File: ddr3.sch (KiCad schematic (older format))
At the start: 17 parts

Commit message: add ddr3
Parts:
- added C? (x7): 0.22u, symbol C
- added C?: 22u, symbol C
- added C? (x4): 2.2p, symbol C
- added R?: 240, symbol R
- added R?: 470, symbol R
- added TP? (x2): A0, symbol TESTPOINT
- added TP? (x2): DQ0, symbol TESTPOINT
- added TP? (x2): CK, symbol TESTPOINT
- added TP? (x2): ~CK, symbol TESTPOINT
- added TP? (x4): GND, symbol TESTPOINT
- added U?: MT41K256M16-107, symbol DDR3-96FBGA
- R?: value Rs -> 10k; symbol Rs -> R
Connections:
- net labels added: DRAM_A0, DRAM_A1, DRAM_A10, DRAM_A11, DRAM_A12, DRAM_A13, DRAM_A14, DRAM_A2, DRAM_A3, DRAM_A4, DRAM_A5, DRAM_A6, DRAM_A7, DRAM_A8, DRAM_A9, DRAM_A[14:0],DRAM_BA[2:0],DRAM_CONTROL, DRAM_BA0, DRAM_BA1, DRAM_BA2, DRAM_CK, DRAM_CKE, DRAM_DATA[15:0],DRAM_DQ,DRAM_DM, DRAM_DQ0, DRAM_DQ1, DRAM_DQ10, DRAM_DQ11, DRAM_DQ12, DRAM_DQ13, DRAM_DQ14, DRAM_DQ15, DRAM_DQ2, DRAM_DQ3, DRAM_DQ4, DRAM_DQ5, DRAM_DQ6, DRAM_DQ7, DRAM_DQ8, DRAM_DQ9, DRAM_LDM, DRAM_LDQS, DRAM_ODT, DRAM_UDM, DRAM_UDQS, ~DRAM_CAS, ~DRAM_CK, ~DRAM_CS, ~DRAM_LDQS, ~DRAM_RAS, ~DRAM_RESET, ~DRAM_UDQS, ~DRAM_WE
- wire segments 38 -> 209
- no-connect marks 0 -> 4
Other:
- note added: "DRAM Termination"
- note added: "DRAM VREF"
- note added: "Signal Integrity"
- note added: "place close to DRAM IC"
- note added: "place close to SoC"
- moved on the sheet: C?, R?, U?B

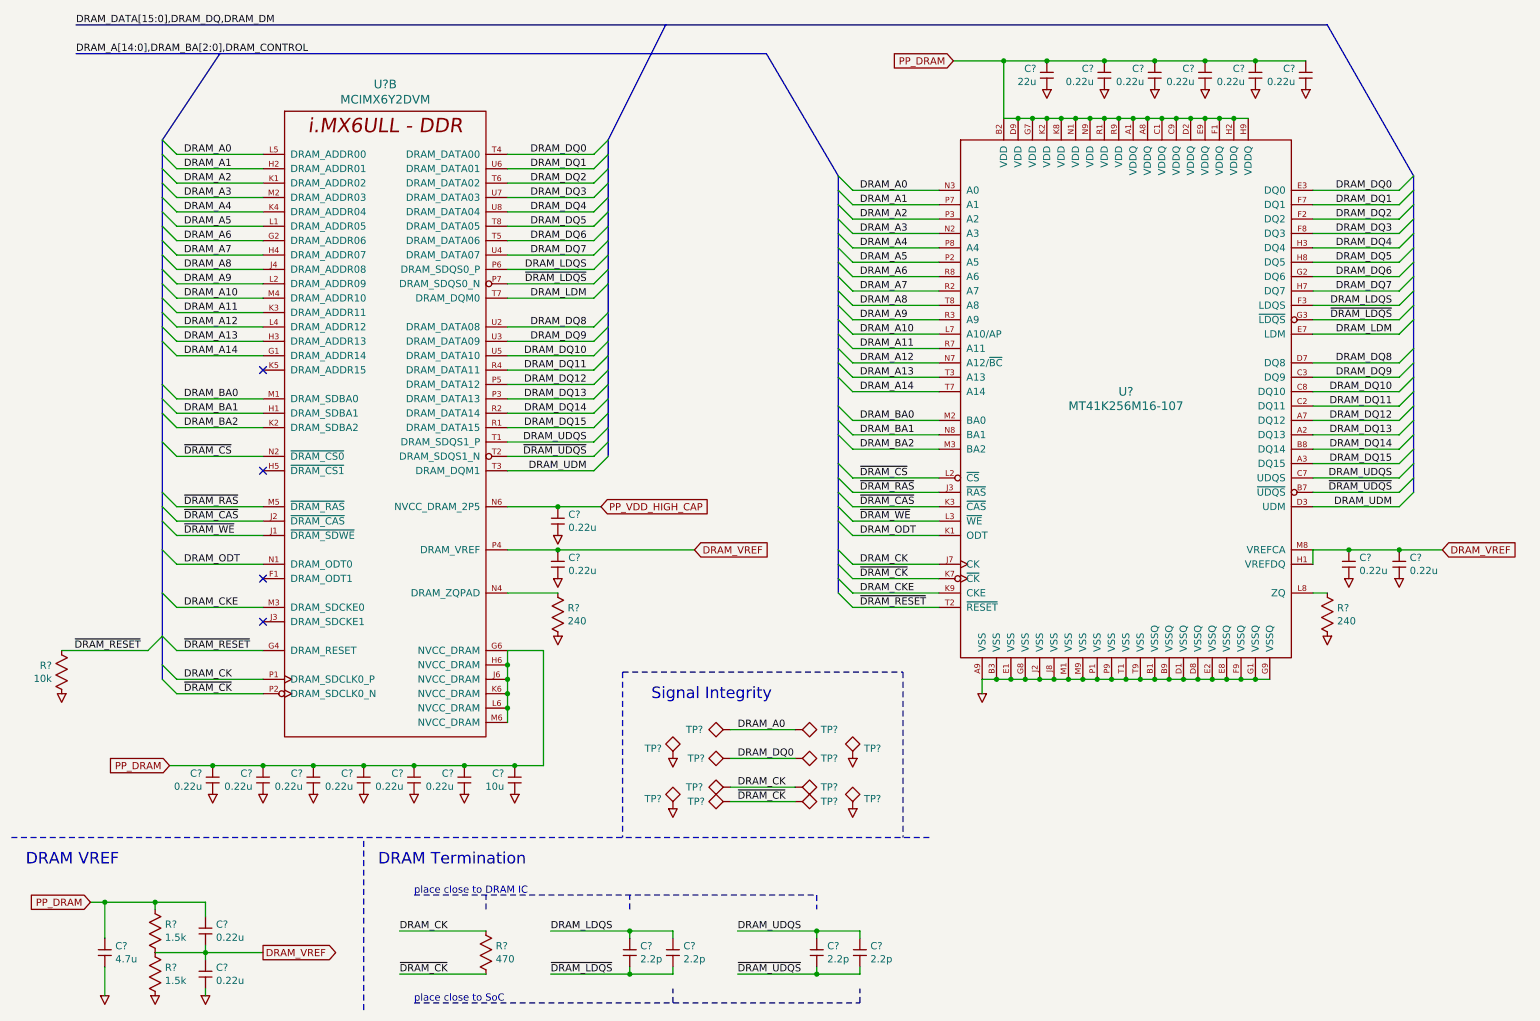
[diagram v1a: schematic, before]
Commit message: ddr, emmc, sd
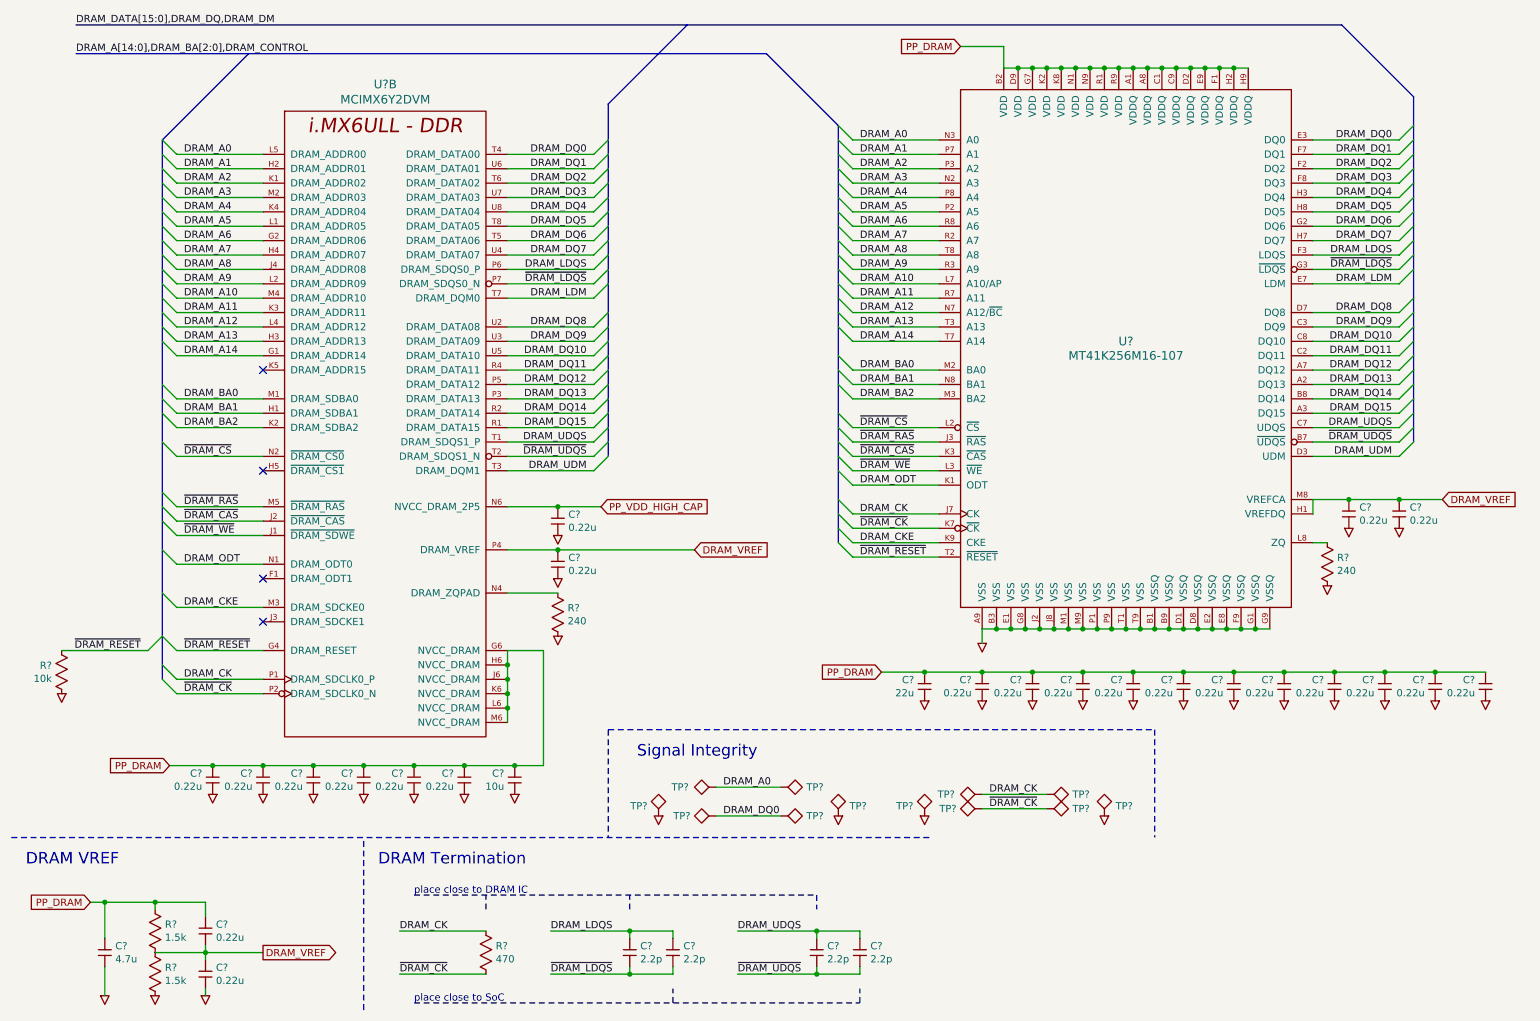
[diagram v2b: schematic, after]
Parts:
- added C? (x6): 0.22u, symbol C
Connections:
- net COM: now also C?.2, C?.2, C?.2, C?.2, C?.2, C?.2
- net PP_DRAM: now also C?.1, C?.1, C?.1, C?.1, C?.1, C?.1
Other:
- moved on the sheet: C?, R?, TP?, U?
